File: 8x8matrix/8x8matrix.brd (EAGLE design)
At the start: 60.4 x 60.5 mm, 18 parts

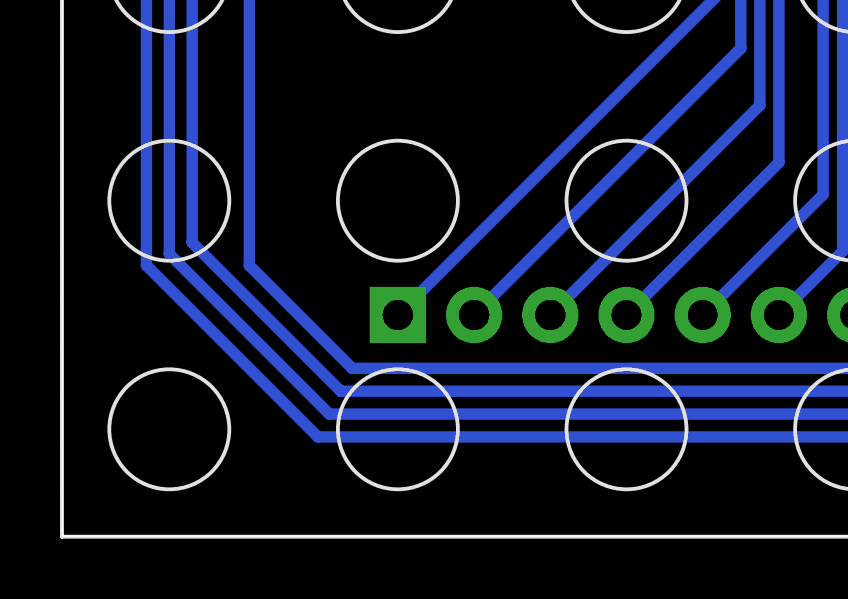
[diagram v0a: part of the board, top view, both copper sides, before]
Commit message: added prints
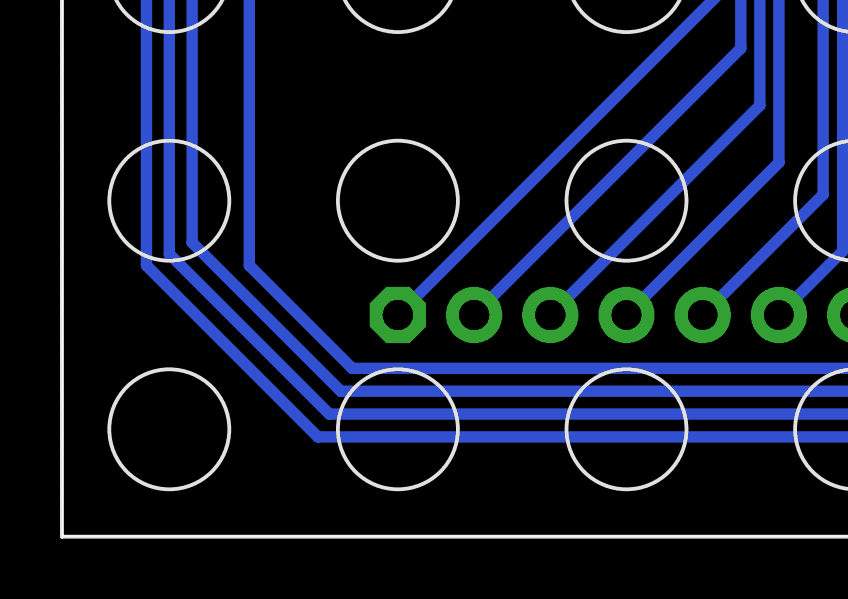
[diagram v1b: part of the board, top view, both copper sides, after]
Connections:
- net N$36 renamed A0
- net N$37 renamed A1
- net N$38 renamed A2
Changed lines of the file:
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@@
 <layer number="20" name="Dimension" color="15" fill="1" visible="yes" active="yes"/>
 <layer number="21" name="tPlace" color="7" fill="1" visible="no" active="yes"/>
-<layer number="22" name="bPlace" color="7" fill="1" visible="no" active="yes"/>
+<layer number="22" name="bPlace" color="7" fill="1" visible="yes" active="yes"/>
 <layer number="23" name="tOrigins" color="15" fill="1" visible="no" active="yes"/>
 <layer number="24" name="bOrigins" color="15" fill="1" visible="yes" active="yes"/>
 <layer number="25" name="tNames" color="7" fill="1" visible="no" active="yes"/>
-<layer number="26" name="bNames" color="7" fill="1" visible="no" active="yes"/>
+<layer number="26" name="bNames" color="7" fill="1" visible="yes" active="yes"/>
 <layer number="27" name="tValues" color="7" fill="1" visible="no" active="yes"/>
-<layer number="28" name="bValues" color="7" fill="1" visible="no" active="yes"/>
+<layer number="28" name="bValues" color="7" fill="1" visible="yes" active="yes"/>
 <layer number="29" name="tStop" color="7" fill="3" visible="no" active="yes"/>
 <layer number="30" name="bStop" color="7" fill="6" visible="no" active="yes"/>
@@
 <layer number="50" name="dxf" color="7" fill="1" visible="no" active="no"/>
 <layer number="51" name="tDocu" color="7" fill="1" visible="no" active="yes"/>
-<layer number="52" name="bDocu" color="7" fill="1" visible="no" active="yes"/>
+<layer number="52" name="bDocu" color="7" fill="1" visible="yes" active="yes"/>
 <layer number="53" name="tGND_GNDA" color="7" fill="9" visible="no" active="no"/>
 <layer number="54" name="bGND_GNDA" color="1" fill="9" visible="no" active="no"/>
@@
 <wire x1="53.252" y1="43.3832" x2="53.594" y2="43.092" width="0.381" layer="16"/>
 </signal>
-<signal name="N$36">
+<signal name="A0">
 <contactref element="U$9" pad="1"/>
 <contactref element="JP2" pad="3"/>
@@
 <wire x1="6.223" y1="9.017" x2="6.223" y2="24.003" width="0.381" layer="16"/>
 </signal>
-<signal name="N$37">
+<signal name="A1">
 <contactref element="U$9" pad="2"/>
 <contactref element="JP2" pad="2"/>
@@
 <wire x1="4.953" y1="25.273" x2="6.223" y2="25.273" width="0.381" layer="16"/>
 </signal>
-<signal name="N$38">
+<signal name="A2">
 <contactref element="U$9" pad="3"/>
 <contactref element="JP2" pad="1"/>
